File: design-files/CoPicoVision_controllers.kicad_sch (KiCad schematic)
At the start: 41 parts, among them J401 Controller 1, J402 Controller 2, Q401 2N3904, Q402 2N3904, U103 74ACT05, U401 74LS541, U402 74LS541, U403 74HCT00

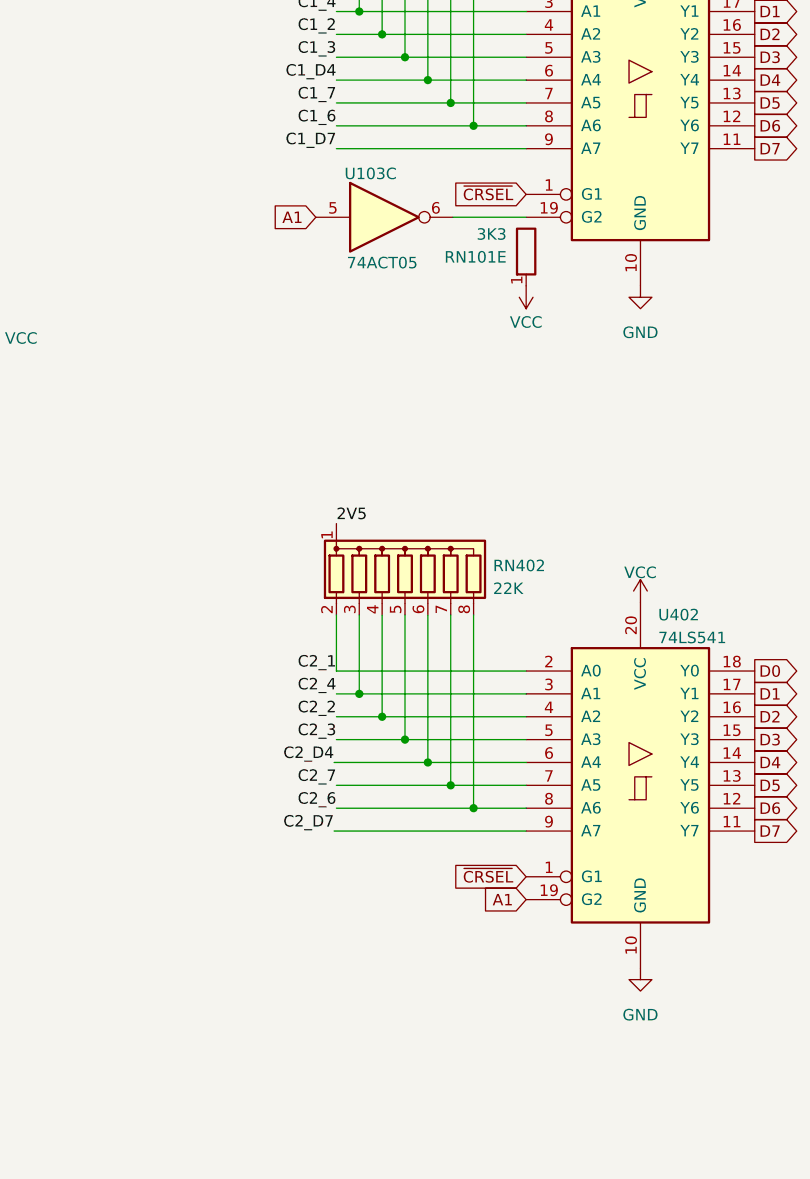
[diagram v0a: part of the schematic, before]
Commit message: Fix the swapped controller problem that rev 0.1 boards have: the G2 input of the 74LS541 is active-low, so A1 low means Controller 1 is selected.
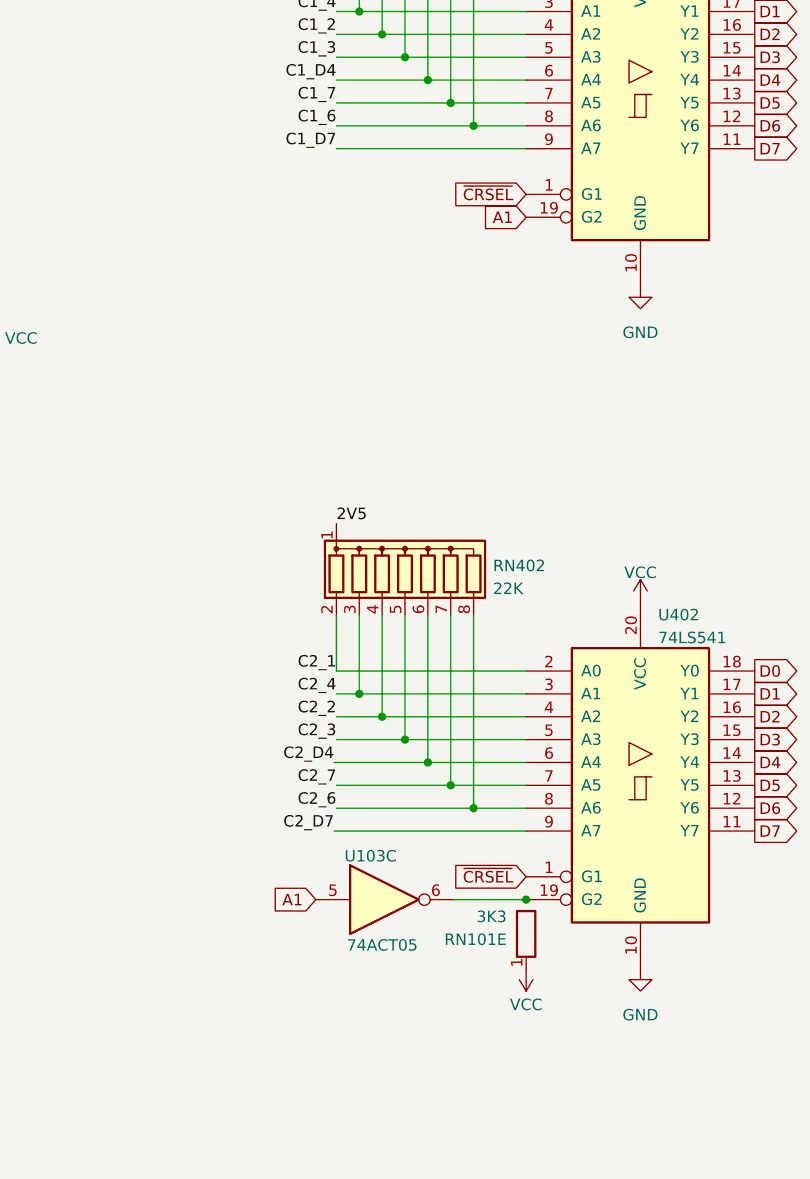
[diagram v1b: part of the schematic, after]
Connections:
- net A1: now also U401.19 (G2); no longer U402.19 (G2)
- net at U103.6: now also U402.19 (G2); no longer U401.19 (G2)
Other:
- moved on the sheet: RN101E, U103C
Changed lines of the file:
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@@
   (title_block
     (title "CoPicoVision")
-    (date "2024-08-31")
-    (rev "0.1")
+    (date "2024-10-12")
+    (rev "0.2")
     (company "(c) 2024 Jason R. Thorpe.  See LICENSE.")
   )
@@
   (junction (at 92.075 56.896) (diameter 0) (color 0 0 0 0)
   )
+  (junction (at 239.903 150.622) (diameter 0) (color 0 0 0 0)
+  )
   (junction (at 63.881 113.284) (diameter 0) (color 0 0 0 0)
   )
@@
     (stroke (width 0) (type default))
   )
-  (wire (pts (xy 231.775 74.803) (xy 239.903 74.803))
+  (wire (pts (xy 231.775 150.622) (xy 239.903 150.622))
     (stroke (width 0) (type default))
   )
@@
     )
   )
-  (global_label "A1" (shape input) (at 239.903 150.622 180) (fields_autoplaced)
+  (global_label "A1" (shape input) (at 239.903 74.803 180) (fields_autoplaced)
     (effects (font (size 1.27 1.27)) (justify right))
-    (property "Intersheetrefs" "${INTERSHEET_REFS}" (at 234.6991 150.622 0)
+    (property "Intersheetrefs" "${INTERSHEET_REFS}" (at 234.6991 74.803 0)
       (effects (font (size 1.27 1.27)) (justify right) hide)
     )
@@
     )
   )
-  (global_label "A1" (shape input) (at 216.535 74.803 180) (fields_autoplaced)
+  (global_label "A1" (shape input) (at 216.535 150.622 180) (fields_autoplaced)
     (effects (font (size 1.27 1.27)) (justify right))
-    (property "Intersheetrefs" "${INTERSHEET_REFS}" (at 211.3311 74.803 0)
+    (property "Intersheetrefs" "${INTERSHEET_REFS}" (at 211.3311 150.622 0)
       (effects (font (size 1.27 1.27)) (justify right) hide)
     )
@@
     )
   )
-  (symbol (lib_id "Device:R_Network04_Split") (at 239.903 78.613 180) (unit 5)
-    (in_bom yes) (on_board yes) (dnp no) (fields_autoplaced)
-    (property "Reference" "RN101" (at 237.744 79.248 0)
-      (effects (font (size 1.27 1.27)) (justify left))
-    )
-    (property "Value" "3K3" (at 237.744 76.708 0)
-      (effects (font (size 1.27 1.27)) (justify left))
-    )
-    (property "Footprint" "Resistor_THT:R_Array_SIP5" (at 241.935 78.613 90)
-      (effects (font (size 1.27 1.27)) hide)
-    )
-    (property "Datasheet" "http://www.vishay.com/docs/31509/csc.pdf" (at 239.903 78.613 0)
-      (effects (font (size 1.27 1.27)) hide)
-    )
-    (property "Mouser" "652-4605M-1LF-3.3K" (at 239.903 78.613 0)
+  (symbol (lib_id "Device:R_Network04_Split") (at 239.903 154.432 180) (unit 5)
+    (in_bom yes) (on_board yes) (dnp no) (fields_autoplaced)
+    (property "Reference" "RN101" (at 237.744 155.067 0)
+      (effects (font (size 1.27 1.27)) (justify left))
+    )
+    (property "Value" "3K3" (at 237.744 152.527 0)
+      (effects (font (size 1.27 1.27)) (justify left))
+    )
+    (property "Footprint" "Resistor_THT:R_Array_SIP5" (at 241.935 154.432 90)
+      (effects (font (size 1.27 1.27)) hide)
+    )
+    (property "Datasheet" "http://www.vishay.com/docs/31509/csc.pdf" (at 239.903 154.432 0)
+      (effects (font (size 1.27 1.27)) hide)
+    )
+    (property "Mouser" "652-4605M-1LF-3.3K" (at 239.903 154.432 0)
       (effects (font (size 1.27 1.27)) hide)
     )
@@
     )
   )
-  (symbol (lib_id "74xx:74LS05") (at 224.155 74.803 0) (unit 3)
+  (symbol (lib_id "74xx:74LS05") (at 224.155 150.622 0) (unit 3)
     (in_bom yes) (on_board yes) (dnp no)
-    (property "Reference" "U103" (at 219.71 69.977 0)
-      (effects (font (size 1.27 1.27)) (justify left))
-    )
-    (property "Value" "74ACT05" (at 219.964 79.883 0)
-      (effects (font (size 1.27 1.27)) (justify left))
-    )
-    (property "Footprint" "Package_DIP:DIP-14_W7.62mm_Socket" (at 224.155 74.803 0)
-      (effects (font (size 1.27 1.27)) hide)
-    )
-    (property "Datasheet" "https://www.ti.com/lit/ds/symlink/cd74act05.pdf" (at 224.155 74.803 0)
-      (effects (font (size 1.27 1.27)) hide)
-    )
-    (property "Mouser" "595-CD74ACT05EE4" (at 224.155 74.803 0)
+    (property "Reference" "U103" (at 219.71 145.796 0)
+      (effects (font (size 1.27 1.27)) (justify left))
+    )
+    (property "Value" "74ACT05" (at 219.964 155.702 0)
+      (effects (font (size 1.27 1.27)) (justify left))
+    )
+    (property "Footprint" "Package_DIP:DIP-14_W7.62mm_Socket" (at 224.155 150.622 0)
+      (effects (font (size 1.27 1.27)) hide)
+    )
+    (property "Datasheet" "https://www.ti.com/lit/ds/symlink/cd74act05.pdf" (at 224.155 150.622 0)
+      (effects (font (size 1.27 1.27)) hide)
+    )
+    (property "Mouser" "595-CD74ACT05EE4" (at 224.155 150.622 0)
       (effects (font (size 1.27 1.27)) hide)
     )
@@
     )
   )
-  (symbol (lib_id "power:VCC") (at 239.903 82.423 180) (unit 1)
-    (in_bom yes) (on_board yes) (dnp no) (fields_autoplaced)
-    (property "Reference" "#PWR0407" (at 239.903 78.613 0)
-      (effects (font (size 1.27 1.27)) hide)
-    )
-    (property "Value" "VCC" (at 239.903 86.487 0)
-      (effects (font (size 1.27 1.27)))
-    )
-    (property "Footprint" "" (at 239.903 82.423 0)
-      (effects (font (size 1.27 1.27)) hide)
-    )
-    (property "Datasheet" "" (at 239.903 82.423 0)
-      (effects (font (size 1.27 1.27)) hide)
-    )
+  (symbol (lib_id "power:VCC") (at 239.903 158.242 180) (unit 1)
+    (in_bom yes) (on_board yes) (dnp no) (fields_autoplaced)
+    (property "Reference" "#PWR0407" (at 239.903 154.432 0)
+      (effects (font (size 1.27 1.27)) hide)
+    )
+    (property "Value" "VCC" (at 239.903 162.306 0)
+      (effects (font (size 1.27 1.27)))
+    )
+    (property "Footprint" "" (at 239.903 158.242 0)
+      (effects (font (size 1.27 1.27)) hide)
+    )
+    (property "Datasheet" "" (at 239.903 158.242 0)
+      (effects (font (size 1.27 1.27)) hide)
+    )
